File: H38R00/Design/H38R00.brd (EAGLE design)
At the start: 34.6 x 60 mm, 38 parts, among them P1 HEXABIT_17.32_X2_POWER_ONLY, U1 LM5160DNT, U2 TPS65130RGERT, X1 INPUT, X2 OUT-15P, X3 OUT-15N, X4 OUT-5P

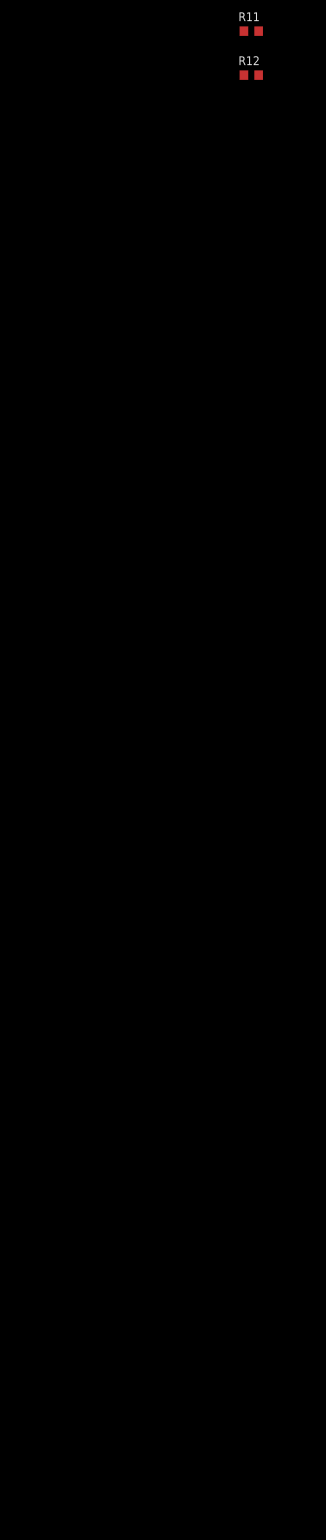
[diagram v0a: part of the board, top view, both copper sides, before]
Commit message: Finished schematics
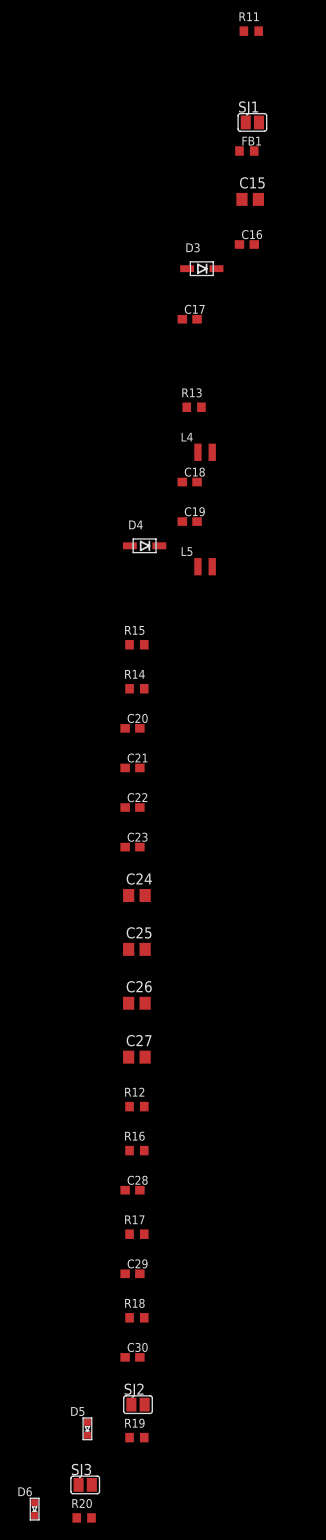
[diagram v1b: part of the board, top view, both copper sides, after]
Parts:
- added C15, C24, C25, C26, C27: 10uF, Hexabitz:C-0805
- added C16, C17, C20, C21: 100nF, Hexabitz:C-0603
- added C18: 4700pF, Hexabitz:C-0603
- added C19: 10nF, Hexabitz:C-0603
- added C22, C23: 1uF, Hexabitz:C-0603
- added C28: 5.6pF, Hexabitz:C-0603
- added C29: 220nF, Hexabitz:C-0603
- added C30: 6.8pF, Hexabitz:C-0603
- added D3, D4: DIOD-SOD-123, Hexabitz:SOD123
- added D5, D6: GREEN, Hexabitz:VLMS1300-GS08
- added FB1: 600 Ohm, Hexabitz:FB-0603
- added L4, L5: 10uH, Hexabitz:WUERTH_ELEKTRONIK_74404024100_0
- added R13: 100.0, Hexabitz:R-0603
- added R14, R15: 1.00, Hexabitz:R-0603
- added R16: 1.30M, Hexabitz:R-0603
- added R17: 86.6K, Hexabitz:R-0603
- added R18: 976K, Hexabitz:R-0603
- added R19, R20: 5.36K, Hexabitz:R-0603
- added SJ1, SJ2, SJ3: (no value), jumper:SJ
- R12: value 0.0 -> 105K
- moved R12 119.9 mm to (-52.7, -286.0)
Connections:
- removed net INN: U2.6
- removed net INN_2: U2.5
- removed net INP: U2.24
- removed net INP_2: U2.1
- removed net OUTN: U2.14
- removed net OUTN_2: U2.13
- removed net PAD: U2.25
- removed net PGND: U2.3
- removed net PGND_2: U2.2
- removed net VIN: U2.4
- new net +15V: C24.1, C25.1, R14.2, SJ2.1, X2.1
- new net +5V: C12.1, C13.1, FB1.1, L3.2, SJ1.1, X4.1
- new net -15V: C26.2, C27.2, R15.2, SJ3.2, X3.2
- new net N$21: D3.1, L4.2, U2.1, U2.24
- new net N$22: C21.1, C23.1, C30.2, D3.2, R14.1, R18.1, U2.23
- new net N$23: C17.1, R13.1, U2.10, U2.11, U2.4, U2.8, U2.9
- new net N$24: C18.1, U2.18
- new net N$25: C19.1, U2.21
- new net N$26: D4.2, L5.1, U2.13, U2.14
- new net N$27: C20.2, C22.2, C28.2, D4.1, R15.1, R16.1, U2.15
- new net N$28: C28.1, R12.1, R16.2, U2.16
- new net N$29: C29.1, R12.2, U2.17
- new net N$30: C30.1, R17.2, R18.2, U2.22
- new net N$31: R19.1, SJ2.2
- new net N$32: D5.A, R19.2
- new net N$33: R20.1, SJ3.1
- new net N$34: D6.C, R20.2
- net AGND: now also C15.2, C16.2, C17.2, C18.2, C19.2, C20.1, C21.2, C22.1, C23.2, C24.2, C25.2, C26.1, C27.1, C29.2, D5.C, D6.A, L5.2, R17.1, U2.2, U2.25, U2.3, X2.2, X3.1
- net N$18: now also C15.1, C16.1, FB1.2, L4.1, R13.2, U2.5, U2.6; no longer C12.1, C13.1, L3.2, R12.1, X4.1
- net N$19: now also SJ1.2; no longer R12.2
